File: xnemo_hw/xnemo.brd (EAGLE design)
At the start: 39.7 x 29 mm, 25 parts, among them J1 MICRO_USB_B_RECEPT, J2 DM3D_MICRO_SD, J3 HEADER_2X5, U1 LTC3559, U2 L3GD20, U3 STM32F405RG, U5 HMC5883L, U6 ADXL345, X1 TXC_7A_XTAL

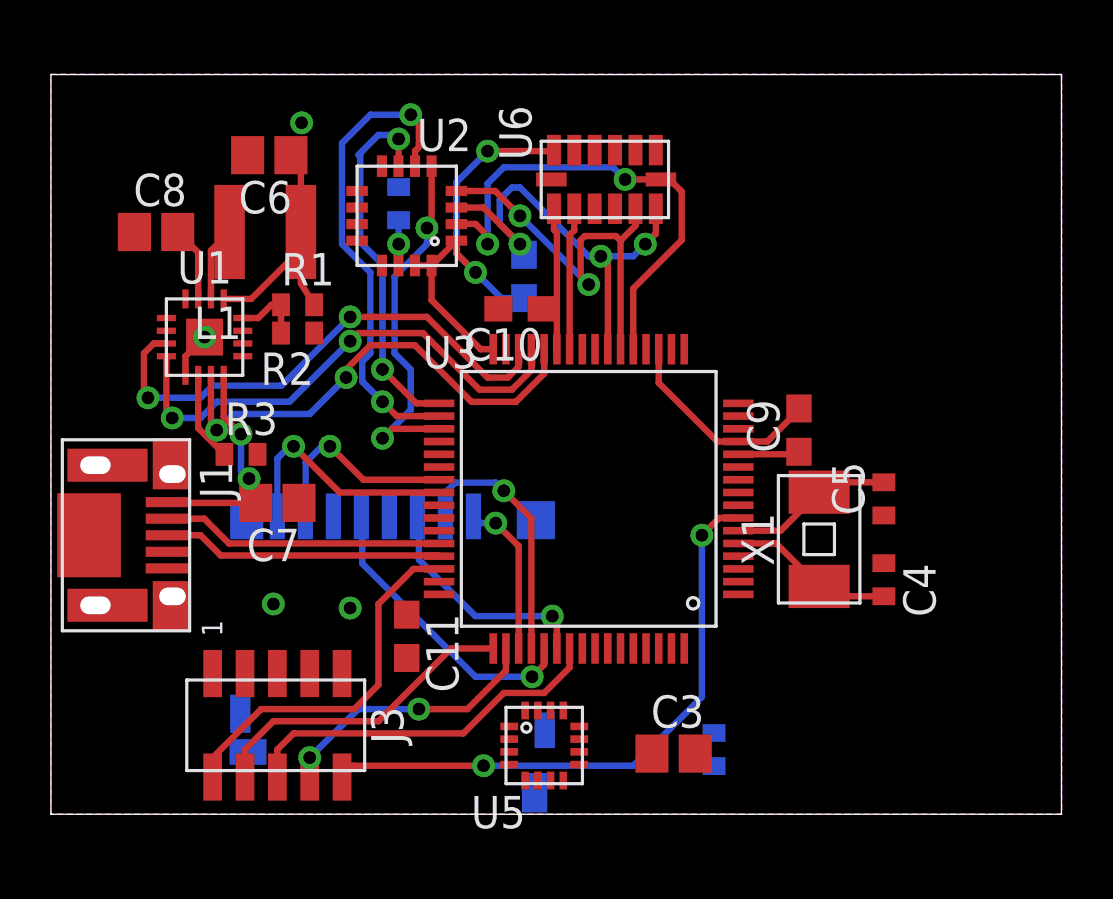
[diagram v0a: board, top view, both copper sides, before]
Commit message: Mostly routed!
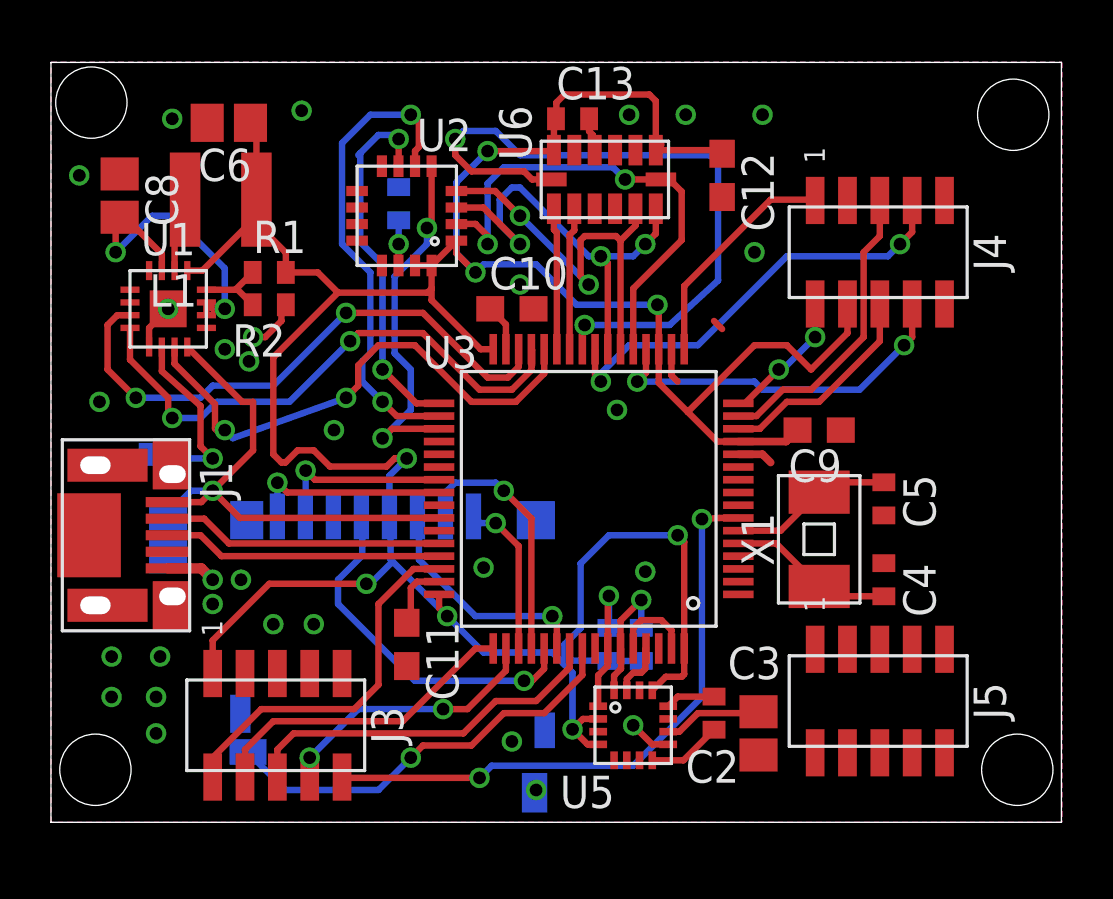
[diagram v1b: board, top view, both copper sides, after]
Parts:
- added C13: 100n, resistor:C0402
- added J4, J5: HEADER_2X5, xnemo:HEADER_2X5_0.05_SMD
- added R5, R6: 22k, resistor:R0402
- moved C12 8.73 mm to (26.4, 25.1), flipped to the top, turned to 270 degrees
- moved C7 4.47 mm to (4.60, 11.0), flipped to the bottom, turned to 90 degrees
- moved U5 3.58 mm to (22.9, 3.49)
- moved C3 3.43 mm to (27.8, 3.17), turned to 270 degrees
- moved R3 3.02 mm to (4.45, 14.1), flipped to the bottom
- moved L1 2.16 mm to (6.67, 24.1)
- moved C6 2.03 mm to (6.99, 27.1)
- moved C8 2.02 mm to (2.70, 24.3), turned to 270 degrees
- moved U1 1.81 mm to (4.60, 19.8)
- moved R1 1.69 mm to (8.57, 21.3)
- moved R2 1.57 mm to (8.57, 20.0)
- moved C2 1.43 mm to (26.0, 3.97), flipped to the top
- moved C9 0.79 mm to (30.2, 15.1), turned to 180 degrees
- moved C11 0.32 mm to (14.0, 6.67)
- moved C10 0.32 mm to (18.1, 19.8), turned to 0 degrees
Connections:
- net N$1 renamed POW_PROG
- removed net JNTRST: U3.P$56
- new net N$1: J5.4
- new net N$15: J4.10
- new net N$16: J5.7
- new net N$17: J5.5
- new net N$2: J5.2
- new net N$3: J5.3
- new net N$4: J5.1
- new net N$5: J5.6
- new net N$6: J5.8
- new net N$7: J4.9
- new net N$8: J5.10
- new net N$9: J5.9
- new net PA0: J4.6, U3.P$14
- new net PA1: J4.5, U3.P$15
- new net PA2: J4.2, U3.P$16
- new net PA3: J4.1, U3.P$17
- new net PA4: J4.8, U3.P$20
- new net PC0: U3.P$8
- new net PC1: U3.P$9
- new net PC2: U3.P$10
- new net PC3: U3.P$11
- new net PC4: J4.7, U3.P$24
- net 3V3: now also C13.1, J4.4, R5.2, R6.2
- net GND: now also C13.2, J4.3, U1.P$9, U3.P$60
- net I2C_SCL: now also R6.1
- net I2C_SDA: now also R5.1
- net MAG_DRDY: now also U3.P$61
- net SD_DET: now also U3.P$56
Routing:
- net 3V3: track 37.7 -> 131.2 mm, vias 2 -> 8
- net SPI_CS_ACC: track 0.00 -> 27.3 mm, vias 0 -> 2
- net PC4: track 0.00 -> 17.4 mm, vias 0 -> 2
- net SD_DET: track 0.00 -> 16.7 mm, vias 0 -> 1
- net PA4: track 0.00 -> 14.5 mm, vias 0 -> 2
- net VUSB: track 8.99 -> 21.1 mm, vias 2 -> 1
- net PA1: track 0.00 -> 11.8 mm
- net GND: track 4.23 -> 15.5 mm, vias 4 -> 30
- net VBAT: track 2.96 -> 13.0 mm, vias 0 -> 2
- net PA3: track 0.00 -> 9.04 mm
- net PA0: track 0.00 -> 8.44 mm
- net I2C_SCL: track 0.00 -> 5.76 mm, vias 0 -> 1
- net PA2: track 0.00 -> 5.39 mm, vias 0 -> 2
- net I2C_SDA: track 0.00 -> 5.10 mm, vias 0 -> 1
- net MAG_C1: track 0.00 -> 3.85 mm
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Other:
- board size 39.7 x 29 mm -> 39.7 x 29.8 mm
